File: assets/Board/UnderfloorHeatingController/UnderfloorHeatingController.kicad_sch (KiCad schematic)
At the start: 18 parts, among them J2 Screw_Terminal_01x03, J3 Screw_Terminal_01x03, K1 G5Q-1A, Q1 BC337, U2 Waveshare_ESP32-S3-Tiny, U5 ACS725LLCTR-10AB-T

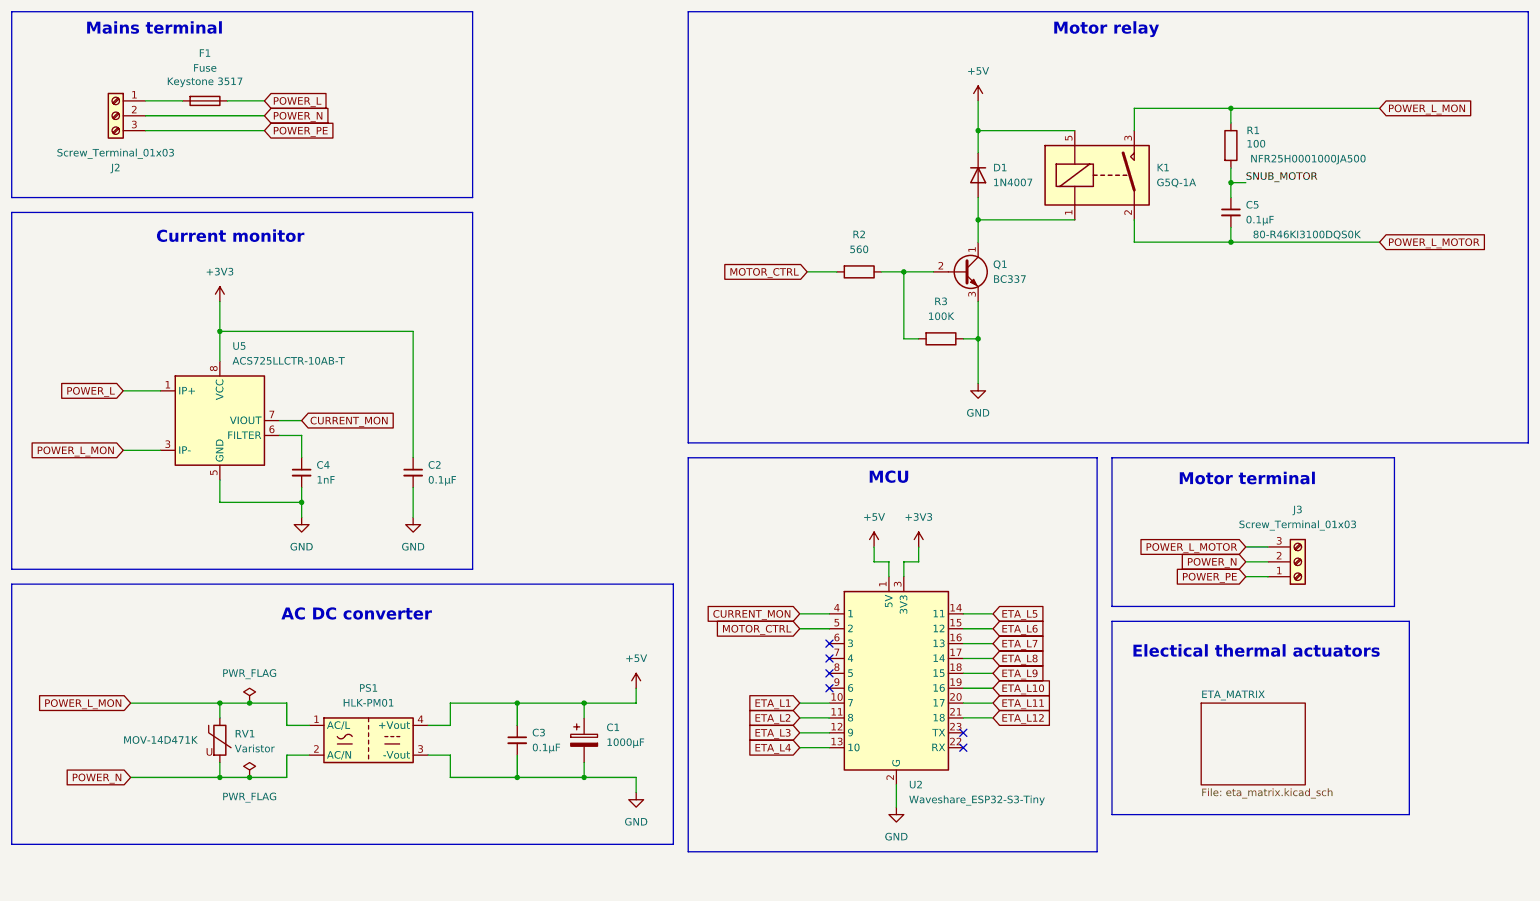
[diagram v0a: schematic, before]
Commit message: First complete design.
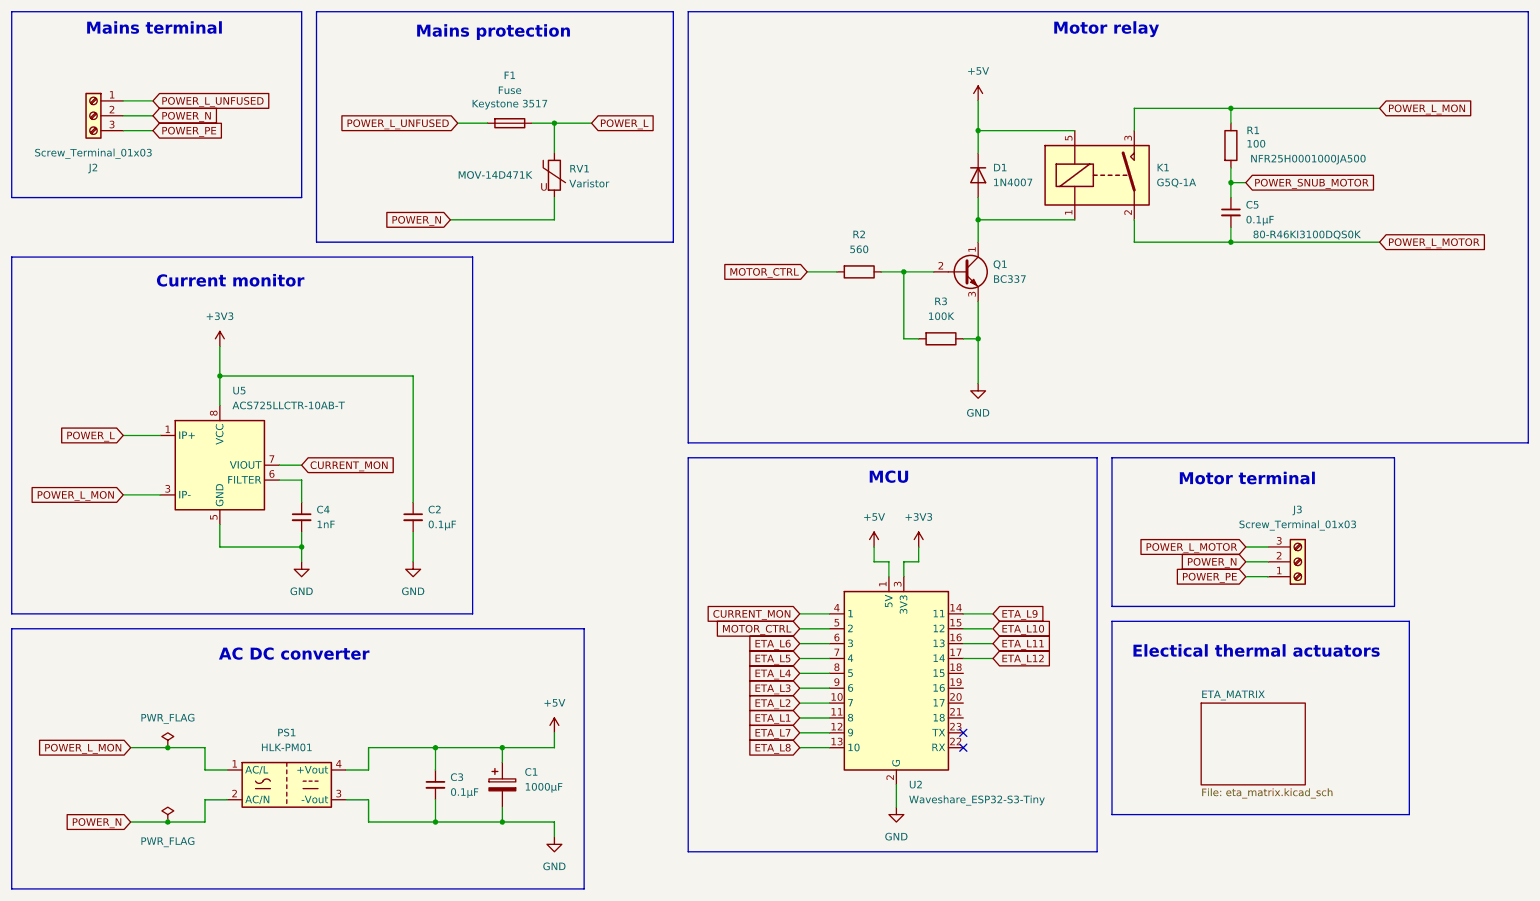
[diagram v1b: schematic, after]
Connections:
- net ETA_L1: now also U2.11 (8); no longer U2.10 (7)
- net ETA_L10: now also U2.15 (12); no longer U2.19 (16)
- net ETA_L11: now also U2.16 (13); no longer U2.20 (17)
- net ETA_L12: now also U2.17 (14); no longer U2.21 (18)
- net ETA_L2: now also U2.10 (7); no longer U2.11 (8)
- net ETA_L3: now also U2.9 (6); no longer U2.12 (9)
- net ETA_L4: now also U2.8 (5); no longer U2.13 (10)
- net ETA_L5: now also U2.7 (4); no longer U2.14 (11)
- net ETA_L6: now also U2.6 (3); no longer U2.15 (12)
- net ETA_L7: now also U2.12 (9); no longer U2.16 (13)
- net ETA_L8: now also U2.13 (10); no longer U2.17 (14)
- net ETA_L9: now also U2.14 (11); no longer U2.18 (15)
- net POWER_L: now also RV1.1
- net POWER_L_MON: no longer RV1.1
- net POWER_L_UNFUSED: now reaches F1.2, J2.1 (Pin_1)
- net SNUB_MOTOR renamed POWER_SNUB_MOTOR
- no-connect marks 6 -> 2
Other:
- note added: "Mains protection"
- moved on the sheet: C1, C2, C3, C4, F1, J2, PS1, RV1, U5
